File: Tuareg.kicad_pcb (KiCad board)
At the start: 4 copper layers, 101.6 x 103.6 mm, 202 parts, among them CON1 ModICE_48, J1 SWD_boctok, P1 VNLD5090e, P2 FAN1100, P3 VNLD5090e, P4 FAN1100, P5 ISO7421D, Q1 BTS3028SDL, Q2 BTS3028SDL, Q3 ISL9V3040, Q4 BTS3028SDL, Q5 ISL9V3040, U1 NCV1117DT, U2 NCV1117ST, U3 MCP6004, U4 MCP6004, U5 LM2903, U6 STM32F410RBTx, U7 24C64, Y1 lfxtal071673, Y2 cx5032ga

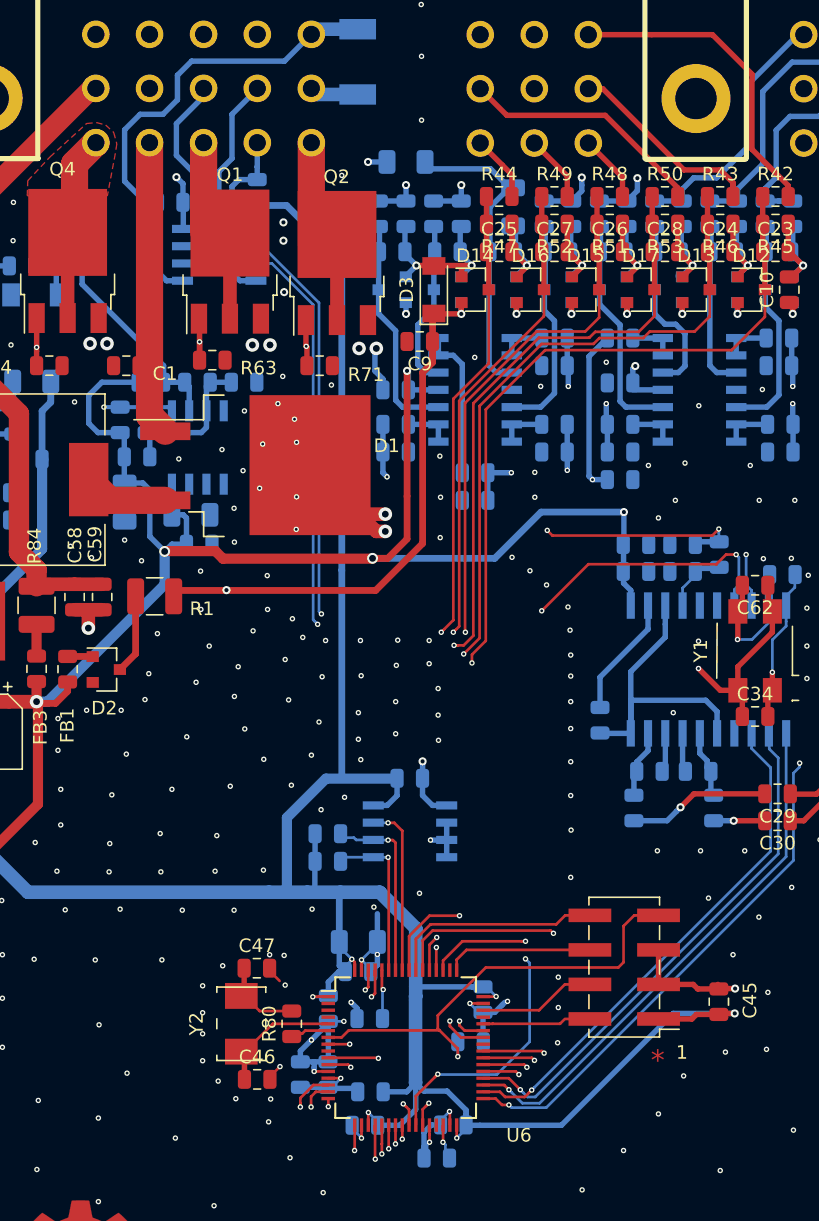
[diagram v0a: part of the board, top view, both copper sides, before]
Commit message: cleaning up bottom layer
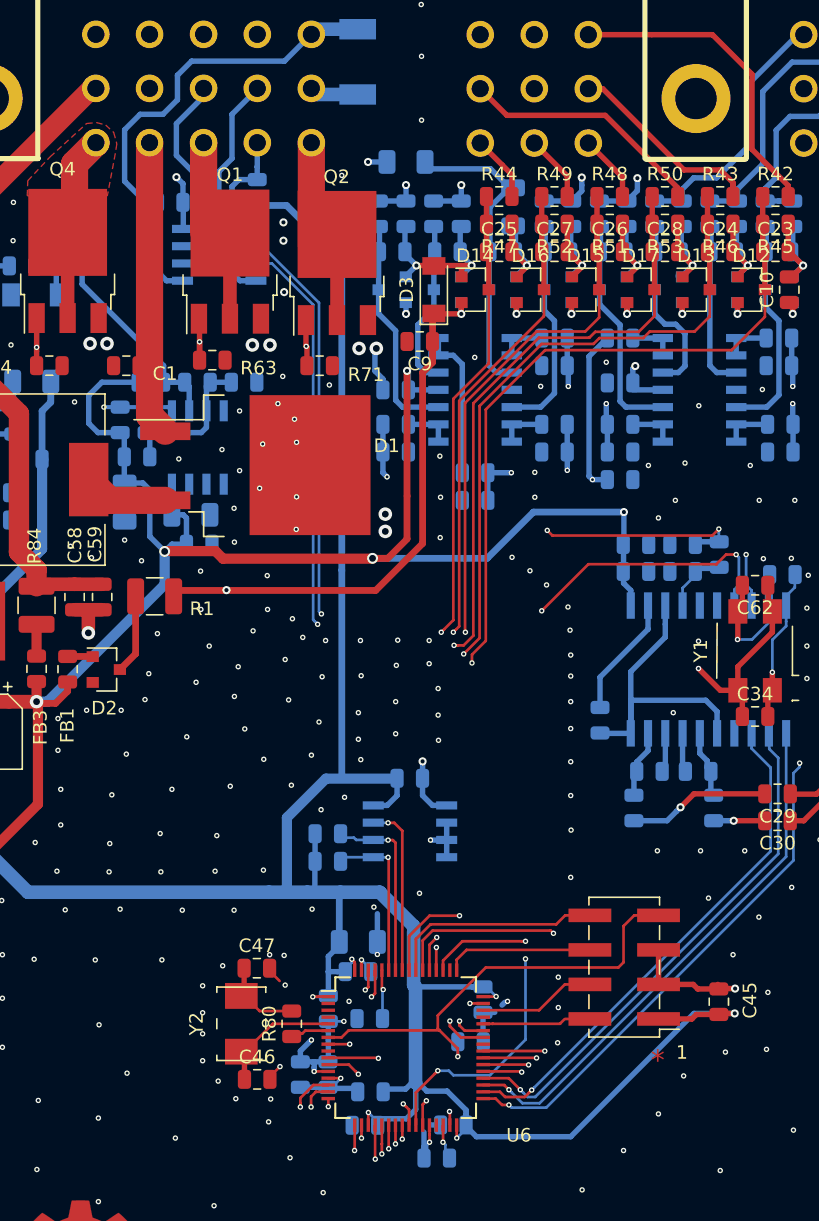
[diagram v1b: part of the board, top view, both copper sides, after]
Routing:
- net GND: track 509.4 -> 471.1 mm
- net /crash: track 83.1 -> 84.2 mm
- net /con_vcci: track 23.2 -> 22.4 mm
- net +3V3: track 213.0 -> 212.3 mm
